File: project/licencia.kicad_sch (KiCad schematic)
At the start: 0 parts

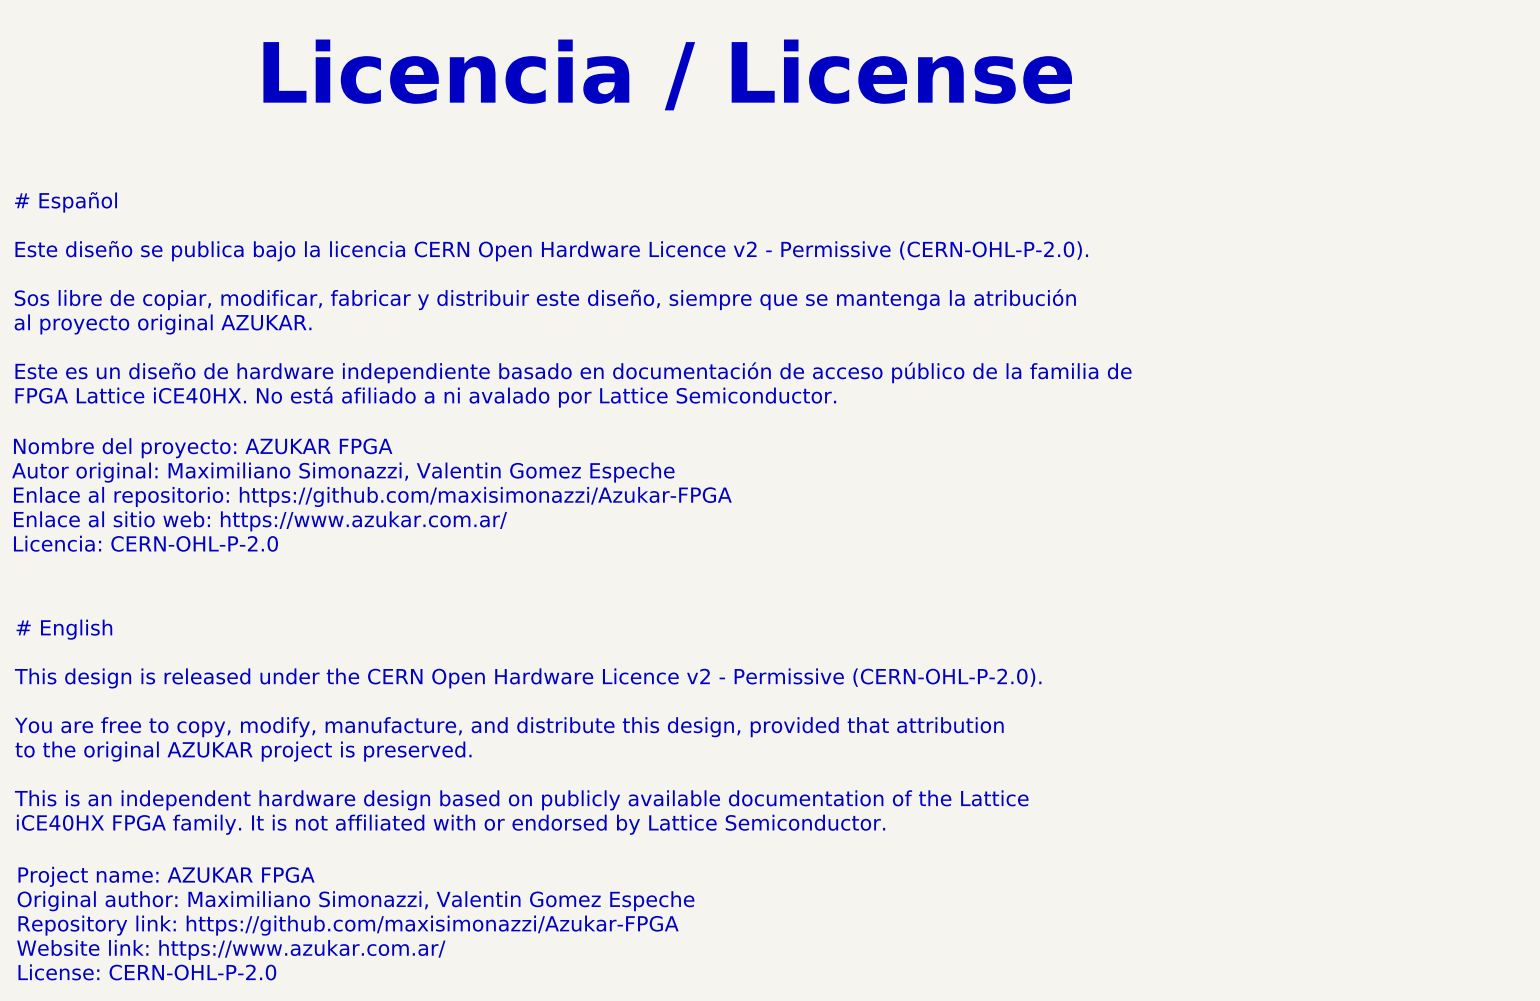
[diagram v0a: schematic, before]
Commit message: pequeño rework a la pcb
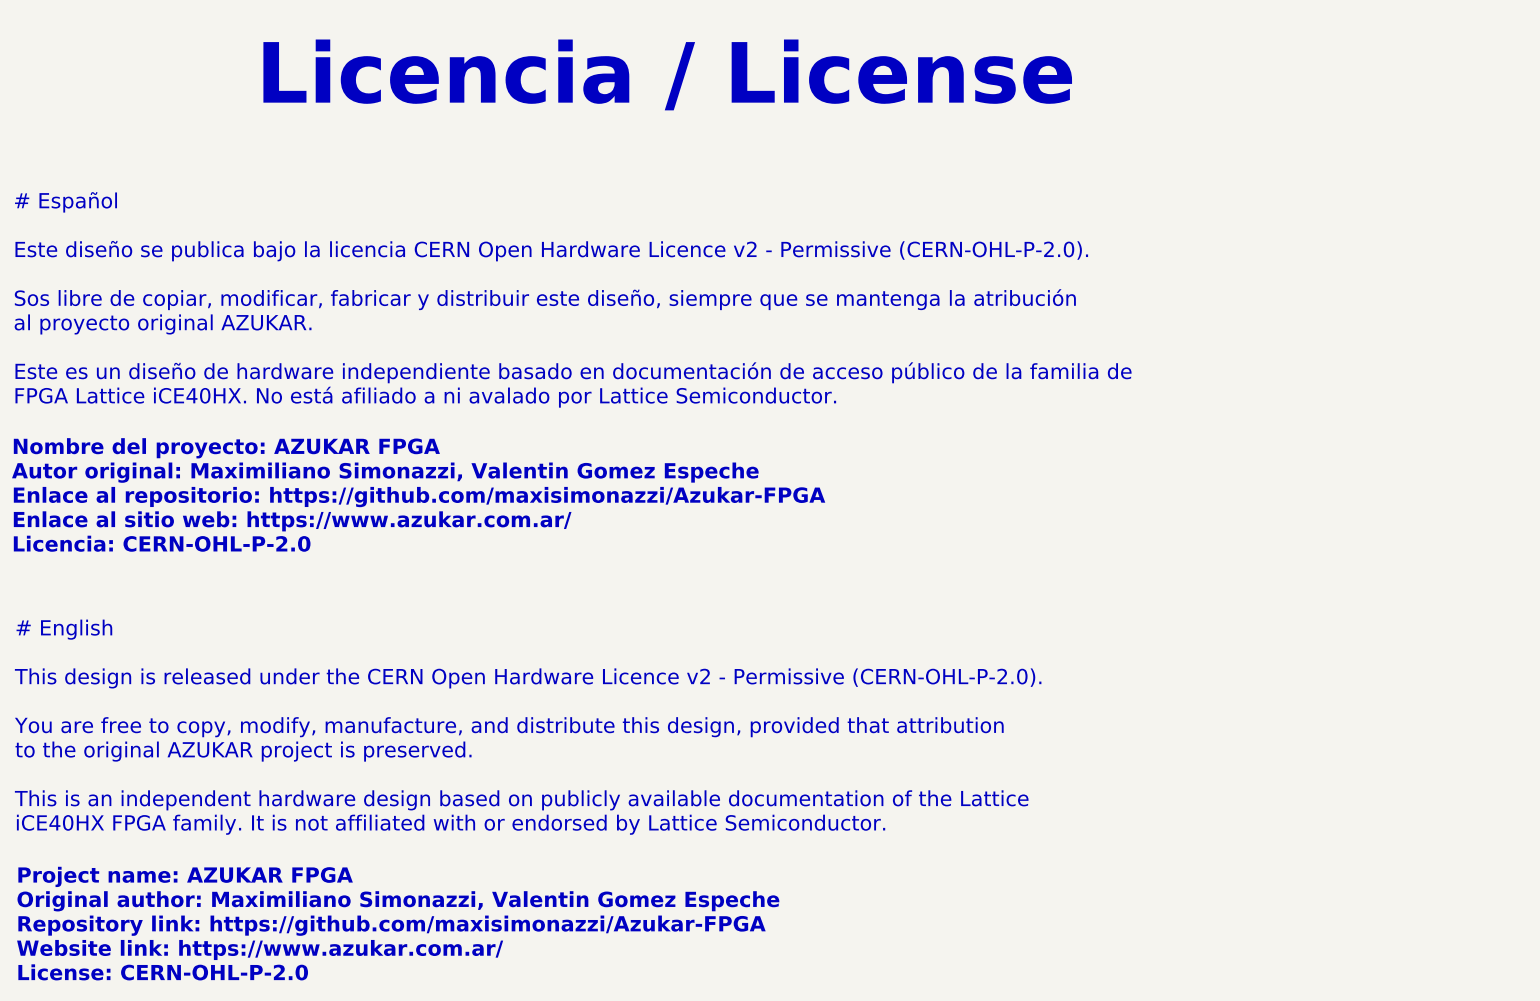
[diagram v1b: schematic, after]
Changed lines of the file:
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@@
 			(font
 				(size 2.54 2.54)
-				(thickness 0.3175)
+				(thickness 0.508)
+				(bold yes)
 			)
 			(justify left)
@@
 			(font
 				(size 2.54 2.54)
+				(thickness 0.508)
+				(bold yes)
 			)
 			(justify left)
